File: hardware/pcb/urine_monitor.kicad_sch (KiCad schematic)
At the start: 25 parts, among them J1 Conn_01x04, J2 GDEY0213B74, J3 USB_C_Receptacle_PowerOnly_6P, Q1 Q_PMOS_GSD, Q2 Q_NMOS_GSD, SW1 SW_Push, U1 RAK3172, U2 HX711, U3 TPS61220DCK, U4 MIC5504-3.3YM5

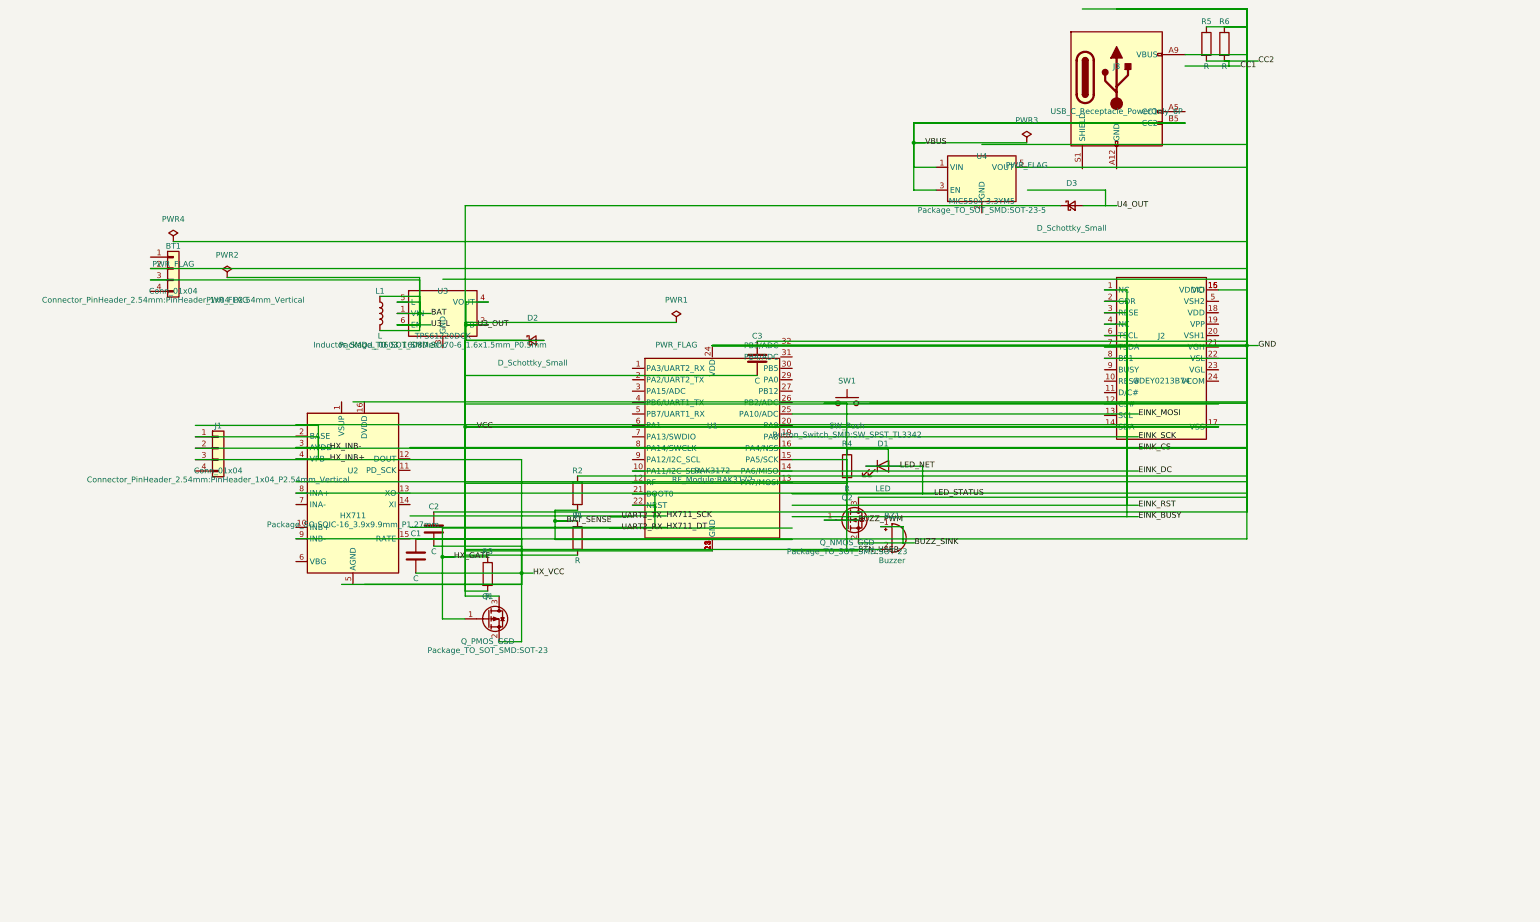
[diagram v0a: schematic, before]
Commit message: init
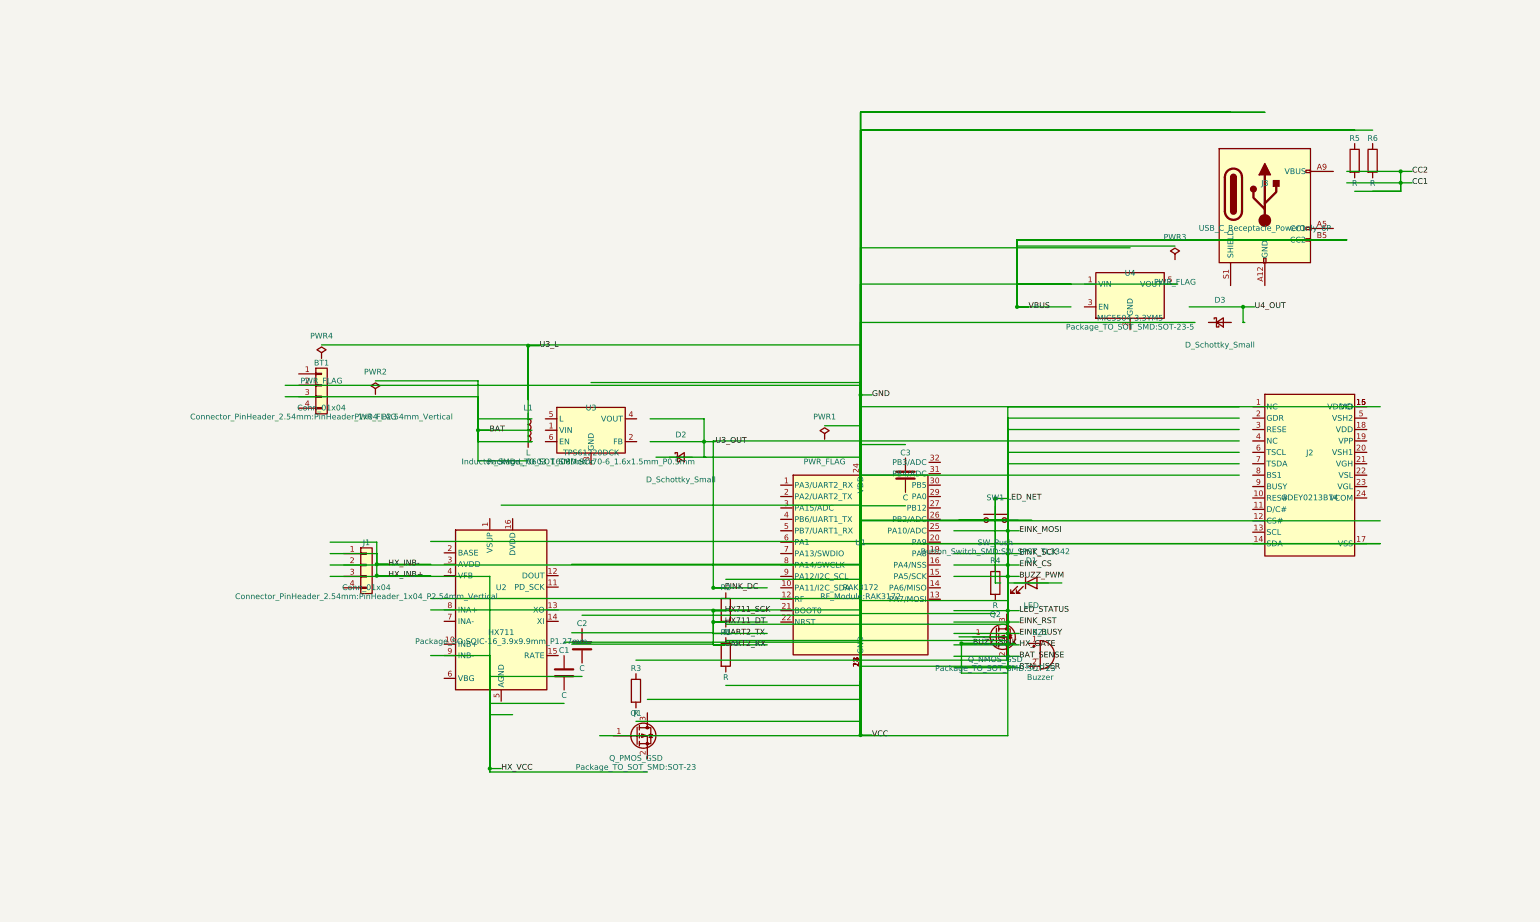
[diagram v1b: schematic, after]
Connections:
- net BAT: no longer BT1.3 (Pin_3), L1.1, L1.2, U3.1 (VIN), U3.5 (L), U3.6 (EN)
- net BAT_SENSE: no longer R1.1, R2.2
- net BUZZ_SINK: no longer BZ1.1 (+), Q2.2 (S)
- net CC1: no longer BT1.2 (Pin_2), C1.1, C2.1, C3.1, J1.2 (Pin_2), J2.1 (NC), J2.15 (VDDIO), J2.16 (VCI), J2.2 (GDR), J2.3 (RESE), J2.4 (NC), J2.6 (TSCL), J2.7 (TSDA), J2.8 (BS1), J3.A9 (VBUS), J3.B9 (VBUS), Q2.3 (D), R2.1, R5.1, R5.2, R6.1, R6.2, SW1.2, U1.10 (PA11/I2C_SDA), U1.16 (PA4/NSS), U1.19 (PA8), U1.24 (VDD), U1.25 (PA10/ADC), U2.8 (INA+)
- net HX711_DT: no longer U1.21 (BOOT0), U1.22 (NRST)
- net HX_INB+: no longer J1.1 (Pin_1), U2.3 (AVDD), U2.4 (VFB)
- net HX_VCC: no longer C1.2, C2.2, J1.3 (Pin_3), Q1.2 (S), U2.9 (INB-)
- net LED_NET: no longer D1.1 (K), R4.1
- net U4_OUT: no longer D3.2 (A)
- removed net BTN_USER: Q2.1 (G), SW1.1, U1.15 (PA5/SCK)
- net HX_GATE: no longer names the net of R3.1
- net HX_GATE: no longer Q1.1 (G)
- net LED_STATUS: no longer names the net of D1.2 (A)
- removed net U3_OUT: BZ1.2 (-), C3.2, D2.1 (K), D2.2 (A), D3.1 (K), J2.17 (VSS), Q1.3 (D), R1.2, R3.2, R4.2, U1.11 (GND), U1.17 (GND), U1.18 (GND), U1.23 (GND), U1.28 (GND), U3.2 (FB), U3.4 (VOUT)
- removed net VBUS: J3.B5 (CC2), U4.1 (VIN), U4.3 (EN)
- new net: J3.A9 (VBUS), J3.B9 (VBUS)
- new net: J2.15 (VDDIO), J2.16 (VCI)
- new net: U1.11 (GND), U1.17 (GND), U1.18 (GND), U1.23 (GND), U1.28 (GND)

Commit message: init
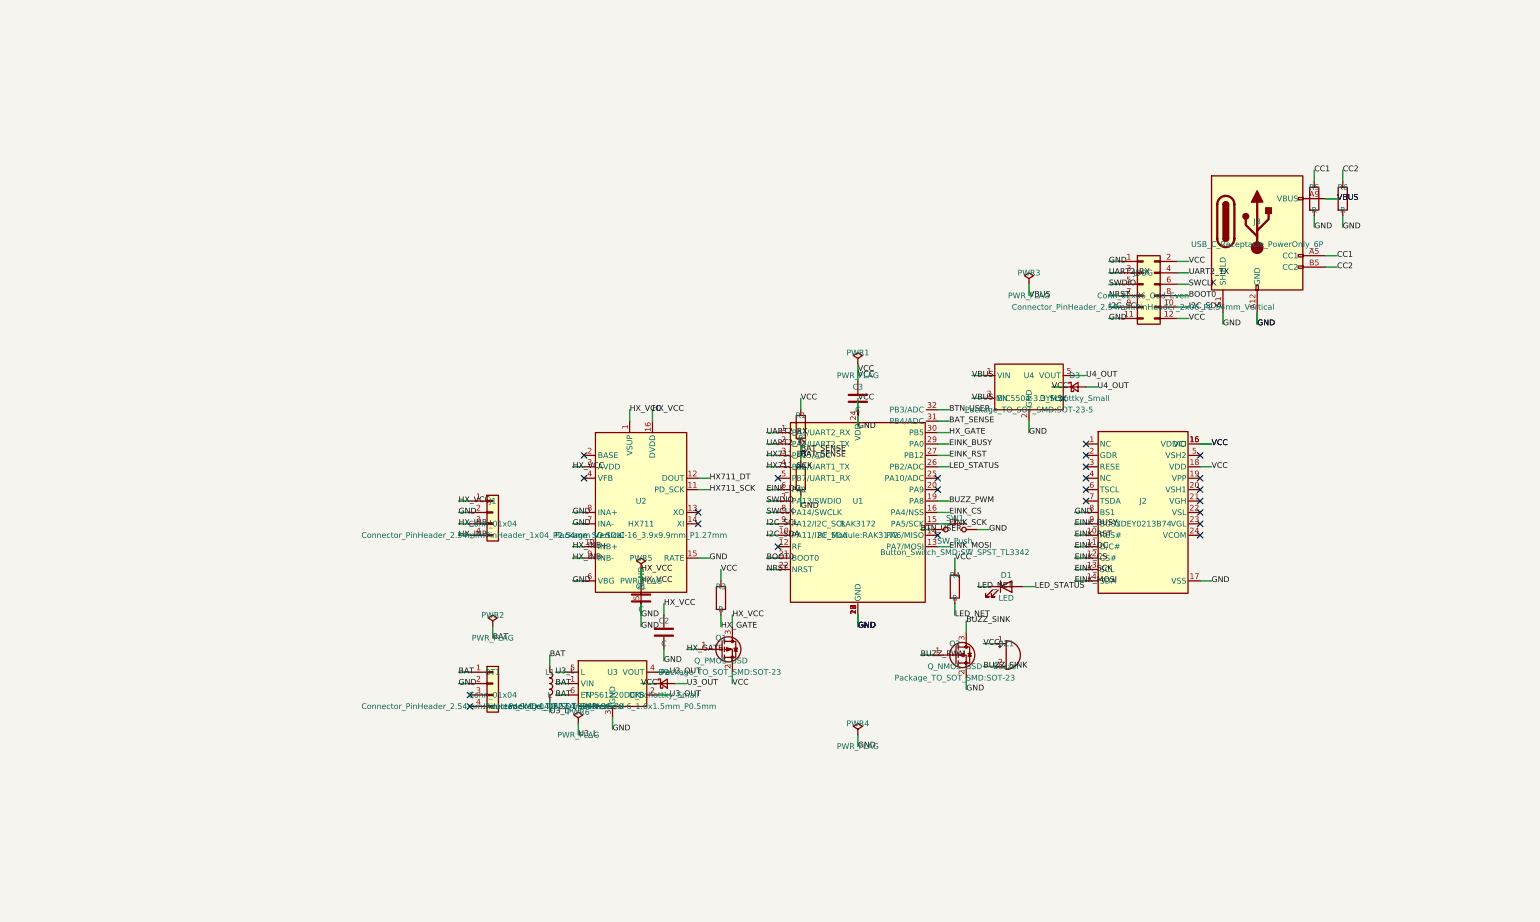
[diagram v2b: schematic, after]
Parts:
- added JDBG: Conn_02x06_Odd_Even, Connector_PinHeader_2.54mm:PinHeader_2x06_P2.54mm_Vertical, symbol Connector_Generic:Conn_02x06_Odd_Even
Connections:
- net BAT: now also BT1.1 (Pin_1), L1.1, U3.1 (VIN), U3.6 (EN)
- net BAT_SENSE: now also R1.2, R2.1, U1.31 (PB4/ADC)
- net BUZZ_SINK: now also BZ1.2 (-), Q2.3 (D)
- net CC1: now also J3.A5 (CC1), R5.1
- net EINK_DC: now also J2.11 (D/C#), U1.6 (PA1)
- net HX711_DT: now also U1.3 (PA15/ADC), U2.12 (DOUT)
- net HX_INB+: now also J1.3 (Pin_3), U2.10 (INB+)
- net HX_VCC: now also C1.1, C2.1, J1.1 (Pin_1), Q1.3 (D), U2.1 (VSUP), U2.16 (DVDD), U2.3 (AVDD)
- net LED_NET: now also D1.1 (K), R4.2
- net U4_OUT: now also D3.2 (A), U4.5 (VOUT)
- net UART2_RX: now also U1.1 (PA3/UART2_RX), JDBG.3 (Pin_3)
- net UART2_TX: now also U1.2 (PA2/UART2_TX), JDBG.4 (Pin_4)
- net LED_STATUS: now reaches D1.2 (A)
- net LED_STATUS: now also U1.26 (PB2/ADC)
- net VCC: now reaches C3.1
- net VCC: now also BZ1.1 (+), D2.1 (K), D3.1 (K), J2.15 (VDDIO), J2.16 (VCI), J2.18 (VDD), Q1.2 (S), R1.1, R3.1, R4.1, U1.24 (VDD), JDBG.12 (Pin_12), JDBG.2 (Pin_2)
- net GND: now reaches C3.2
- net GND: now also BT1.2 (Pin_2), C1.2, C2.2, J1.2 (Pin_2), J2.17 (VSS), J2.8 (BS1), J3.A12 (GND), J3.B12 (GND), J3.S1 (SHIELD), Q2.2 (S), R2.2, R5.2, R6.2, SW1.2, U1.11 (GND), U1.17 (GND), U1.18 (GND), U1.23 (GND), U1.28 (GND), U2.15 (RATE), U2.5 (AGND), U2.6 (VBG), U2.7 (INA-), U2.8 (INA+), U3.3 (GND), U4.2 (GND), JDBG.1 (Pin_1), JDBG.11 (Pin_11)
- net HX_GATE: now reaches R3.2
- net HX_GATE: now also Q1.1 (G), U1.30 (PB5)
- net VBUS: now reaches J3.A9 (VBUS), J3.B9 (VBUS)
- net VBUS: now also U4.1 (VIN), U4.3 (EN)
- net CC2: now reaches J3.B5 (CC2)
- net CC2: now also R6.1
- net U3_OUT: now reaches D2.2 (A)
- net U3_OUT: now also U3.2 (FB), U3.4 (VOUT)
- net HX711_SCK: now reaches U2.11 (PD_SCK)
- net HX711_SCK: now also U1.4 (PB6/UART1_TX)
- net HX_INB-: now reaches U2.9 (INB-)
- net HX_INB-: now also J1.4 (Pin_4)
- net BUZZ_PWM: now reaches Q2.1 (G)
- net BUZZ_PWM: now also U1.19 (PA8)
- net U3_L: now reaches U3.5 (L)
- net U3_L: now also L1.2
- net EINK_RST: now reaches J2.10 (RES#)
- net EINK_RST: now also U1.27 (PB12)
- net EINK_CS: now reaches J2.12 (CS#)
- net EINK_CS: now also U1.16 (PA4/NSS)
- net EINK_SCK: now reaches J2.13 (SCL)
- net EINK_SCK: now also U1.15 (PA5/SCK)
- net EINK_MOSI: now reaches J2.14 (SDA)
- net EINK_MOSI: now also U1.13 (PA7/MOSI)
- net EINK_BUSY: now reaches J2.9 (BUSY)
- net EINK_BUSY: now also U1.29 (PA0)
- net BTN_USER: now reaches SW1.1
- net BTN_USER: now also U1.32 (PB3/ADC)
- net I2C_SDA: now reaches U1.10 (PA11/I2C_SDA)
- net I2C_SDA: now also JDBG.10 (Pin_10)
- net BOOT0: now reaches U1.21 (BOOT0)
- net BOOT0: now also JDBG.8 (Pin_8)
- net NRST: now reaches U1.22 (NRST)
- net NRST: now also JDBG.7 (Pin_7)
- net SWDIO: now reaches U1.7 (PA13/SWDIO)
- net SWDIO: now also JDBG.5 (Pin_5)
- net SWCLK: now reaches U1.8 (PA14/SWCLK)
- net SWCLK: now also JDBG.6 (Pin_6)
- net I2C_SCL: now reaches U1.9 (PA12/I2C_SCL)
- net I2C_SCL: now also JDBG.9 (Pin_9)
- no-connect marks 0 -> 25

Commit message: init
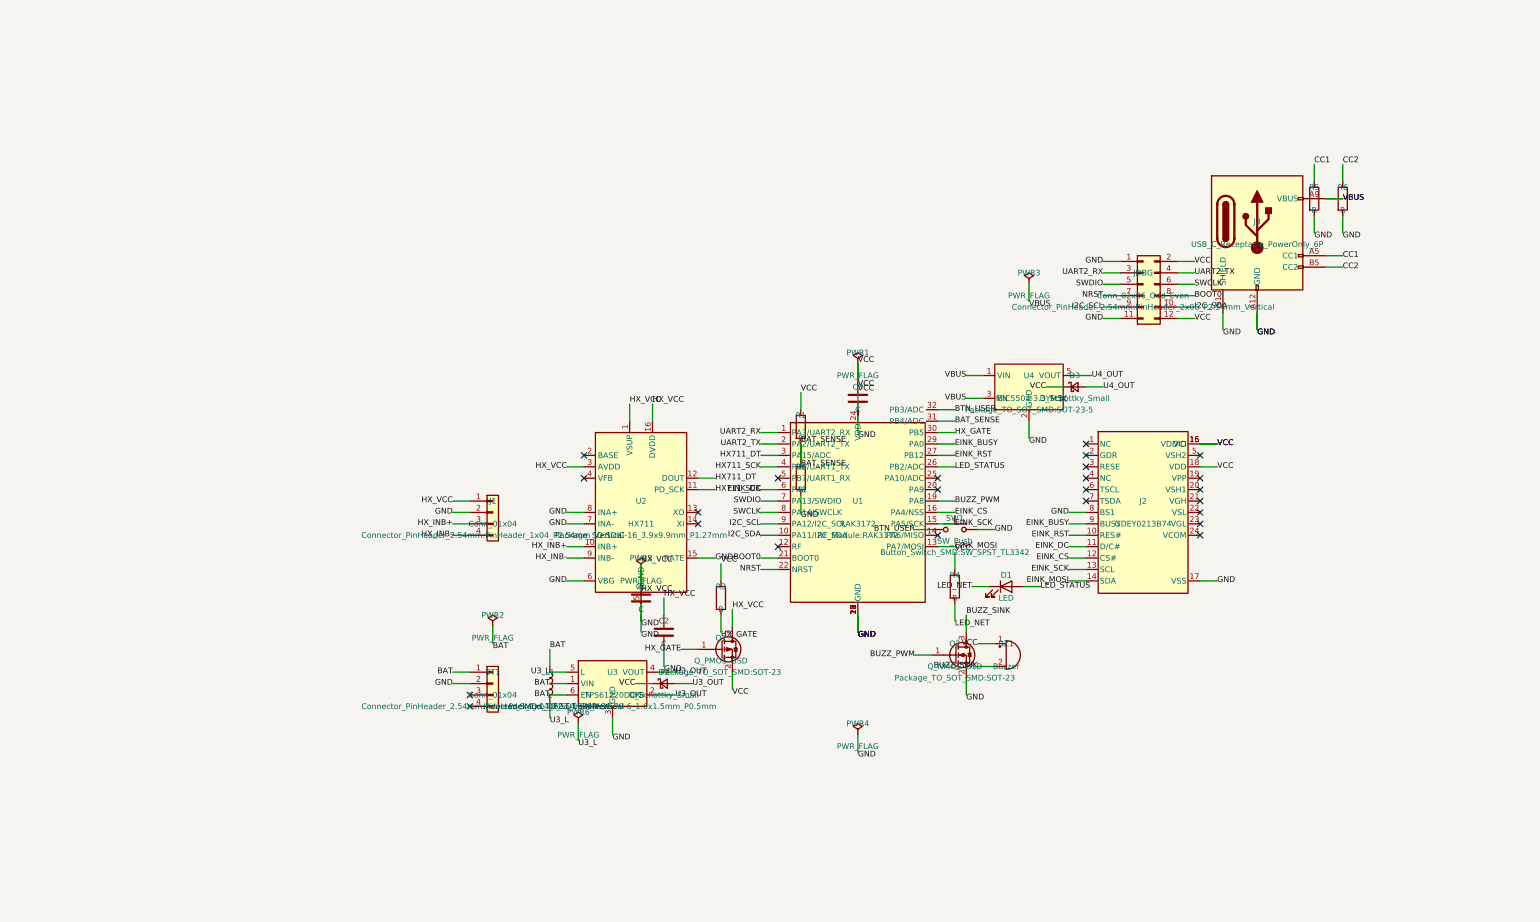
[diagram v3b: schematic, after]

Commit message: init
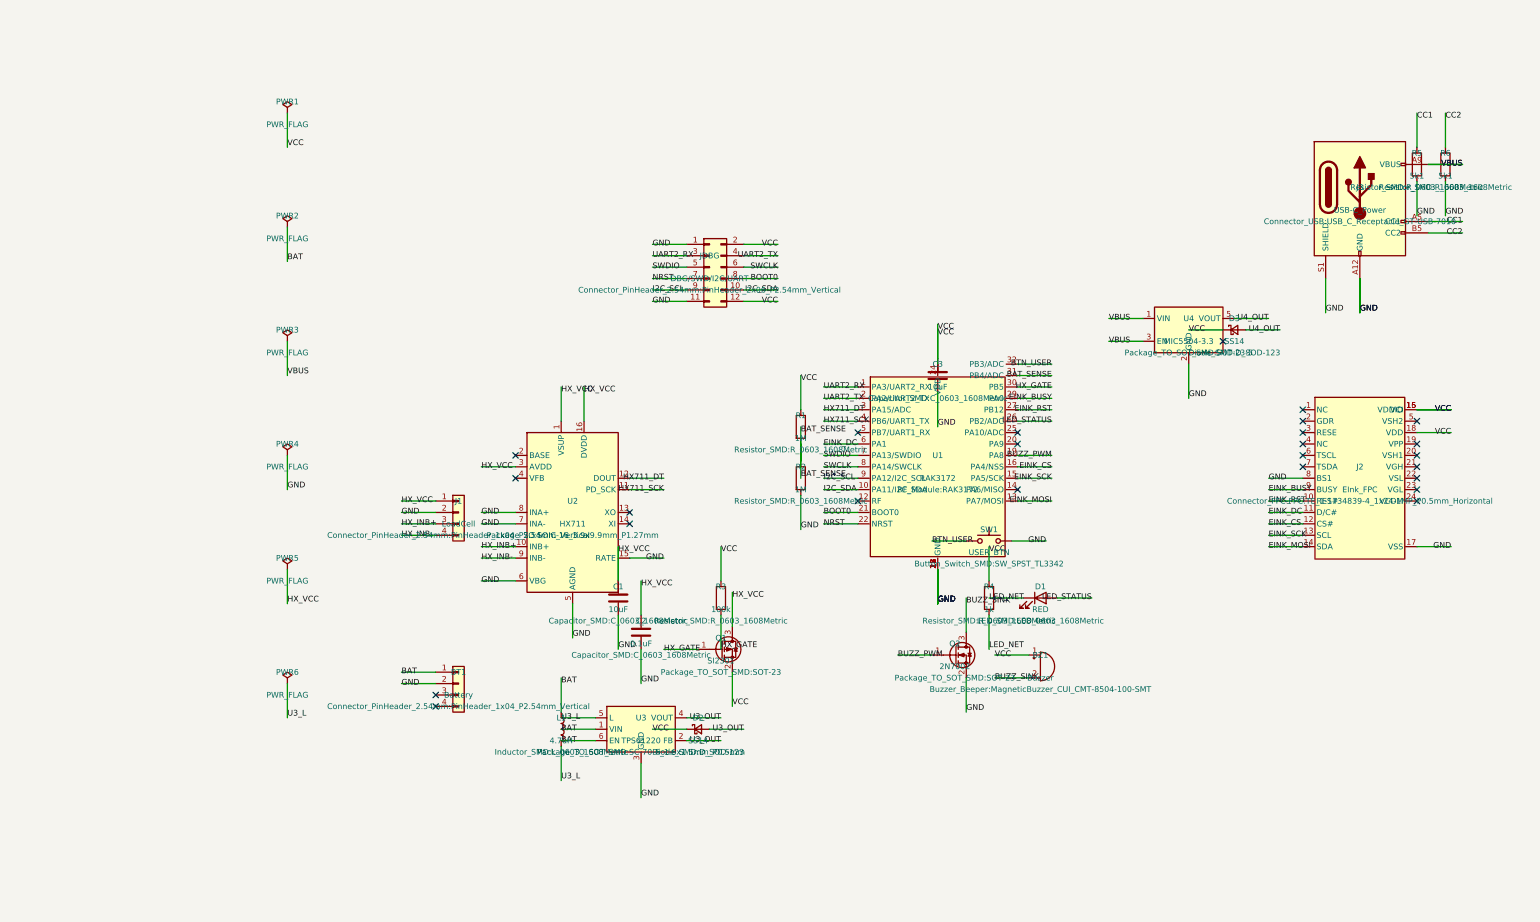
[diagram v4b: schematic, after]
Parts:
- BT1: value Conn_01x04 -> Battery
- BZ1: footprint (none) -> Buzzer_Beeper:MagneticBuzzer_CUI_CMT-8504-100-SMT
- C1, C3: value C -> 10uF; footprint (none) -> Capacitor_SMD:C_0603_1608Metric
- C2: value C -> 0.1uF; footprint (none) -> Capacitor_SMD:C_0603_1608Metric
- D1: value LED -> RED; footprint (none) -> LED_SMD:LED_0603_1608Metric
- D2, D3: value D_Schottky_Small -> SS14; footprint (none) -> Diode_SMD:D_SOD-123
- J1: value Conn_01x04 -> LoadCell
- J2: value GDEY0213B74 -> EInk_FPC; footprint (none) -> Connector_FFC-FPC:TE_1-1734839-4_1x24-1MP_P0.5mm_Horizontal
- J3: value USB_C_Receptacle_PowerOnly_6P -> USB-C_Power; footprint (none) -> Connector_USB:USB_C_Receptacle_GT-USB-7010
- JDBG: value Conn_02x06_Odd_Even -> DBG/SWD/I2C/UART
- L1: value L -> 4.7uH
- Q1: value Q_PMOS_GSD -> SI2301
- Q2: value Q_NMOS_GSD -> 2N7002
- R1, R2: value R -> 1M; footprint (none) -> Resistor_SMD:R_0603_1608Metric
- R3: value R -> 100k; footprint (none) -> Resistor_SMD:R_0603_1608Metric
- R4: value R -> 1k; footprint (none) -> Resistor_SMD:R_0603_1608Metric
- R5, R6: value R -> 5k1; footprint (none) -> Resistor_SMD:R_0603_1608Metric
- SW1: value SW_Push -> USER_BTN
- U3: value TPS61220DCK -> TPS61220
- U4: value MIC5504-3.3YM5 -> MIC5504-3.3
